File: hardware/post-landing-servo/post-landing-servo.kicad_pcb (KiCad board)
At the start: 2 copper layers, 61 x 31.8 mm, 9 parts, among them J1 Conn_01x08, J10 DE9_Socket, J4 Conn_01x08, J6 Conn_01x06, J9 DE9_Socket

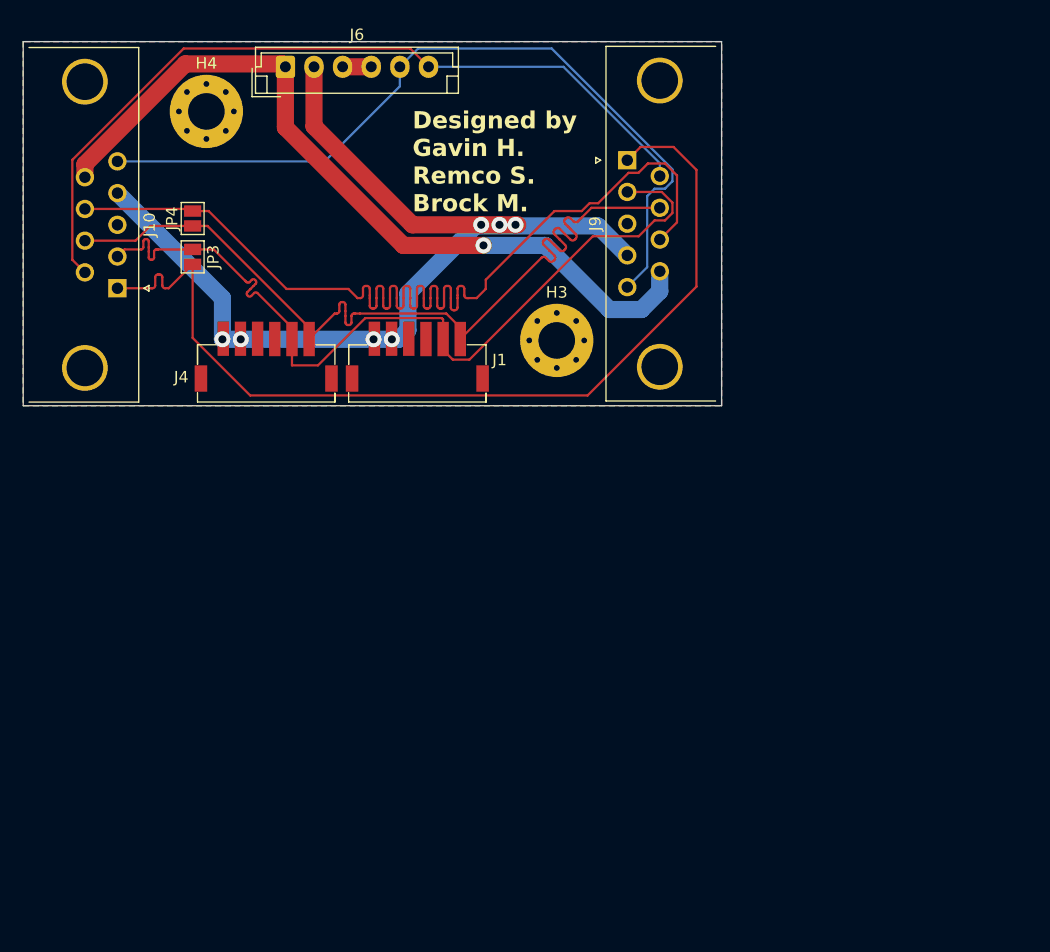
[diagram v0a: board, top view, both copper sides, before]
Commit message: Feat: Reroute and minor fixes
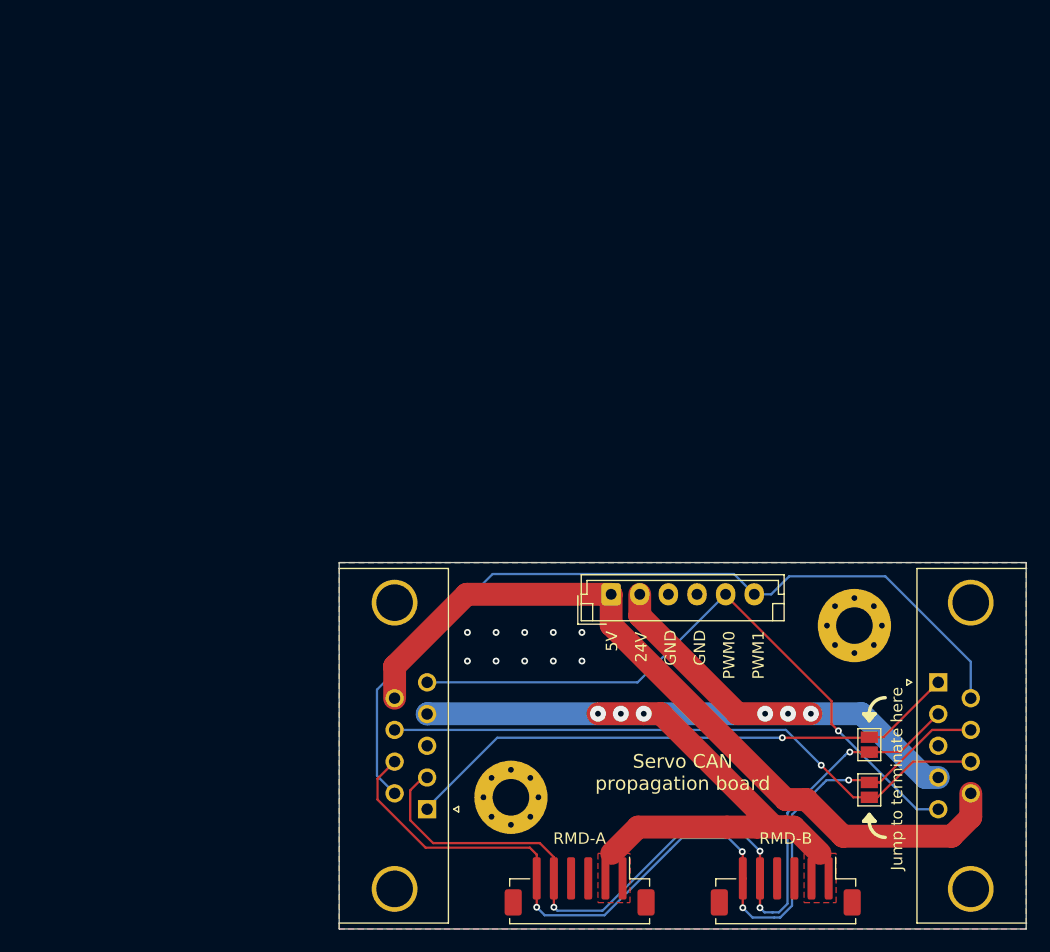
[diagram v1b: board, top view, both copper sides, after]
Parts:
- removed J1, J4: Conn_01x08, Custom:ZH-6PWB_knockoff
- removed J6: Conn_01x06, Connector_JST:JST_EH_B6B-EH-A_1x06_P2.50mm_Vertical
- added 5V    24V   GND    PWM1 PWM2: Conn_01x06, Connector_JST:JST_EH_B6B-EH-A_1x06_P2.50mm_Vertical, F.Cu at (123.8, 102.3)
- added RMD-A: Conn_01x06, Connector_JST:JST_ZH_B6B-ZR-SM4-TF_1x06-1MP_P1.50mm_Vertical, F.Cu at (121.0, 127.8)
- added RMD-B: Conn_01x06, Connector_JST:JST_ZH_B6B-ZR-SM4-TF_1x06-1MP_P1.50mm_Vertical, F.Cu at (139.0, 127.8)
- moved JP4 77.3 mm to (146.3, 119.3), turned to -90 degrees
- moved JP3 72.9 mm to (146.3, 115.4), turned to 90 degrees
- moved H4 72.2 mm to (145.0, 105.0)
- moved J9 53.1 mm to (152.3, 110.0)
- moved J10 52.9 mm to (107.7, 121.0)
- moved H3 40.1 mm to (115.0, 120.0)
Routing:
- net /CAN_B+: track 93.4 -> 54.4 mm, vias 0 -> 1
- net /CAN_B-: track 83.4 -> 49.8 mm, vias 0 -> 1
- net +24V: track 85.5 -> 107.9 mm, vias 7 -> 6
- net /SIG1: track 70.4 -> 56.8 mm, vias 0 -> 1
- net /CAN_A+: track 75.4 -> 85.4 mm, vias 0 -> 4
- net GND: track 2.50 -> 0.00 mm, vias 0 -> 10
- net /SIG2: track 70.9 -> 73.4 mm
- net /CAN_A-: track 75.5 -> 77.9 mm, vias 0 -> 4
- net +5V: track 69.4 -> 68.8 mm, vias 1 -> 0
- added copper zone on F.Cu, net +24V
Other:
- board size 61 x 31.8 mm -> 60 x 32 mm
- board text added: "24V"
- board text added: "5V"
- board text added: "GND"
- board text added: "I should be in a case! Please?"
- board text added: "Jump to terminate here"
- board text added: "PWM0"
- board text added: "PWM1"
- board text added: "Servo CAN propagation board"
- board text removed: "Designed by Gavin H. Remco S. Brock M."
